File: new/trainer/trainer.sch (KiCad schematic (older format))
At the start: 14 parts

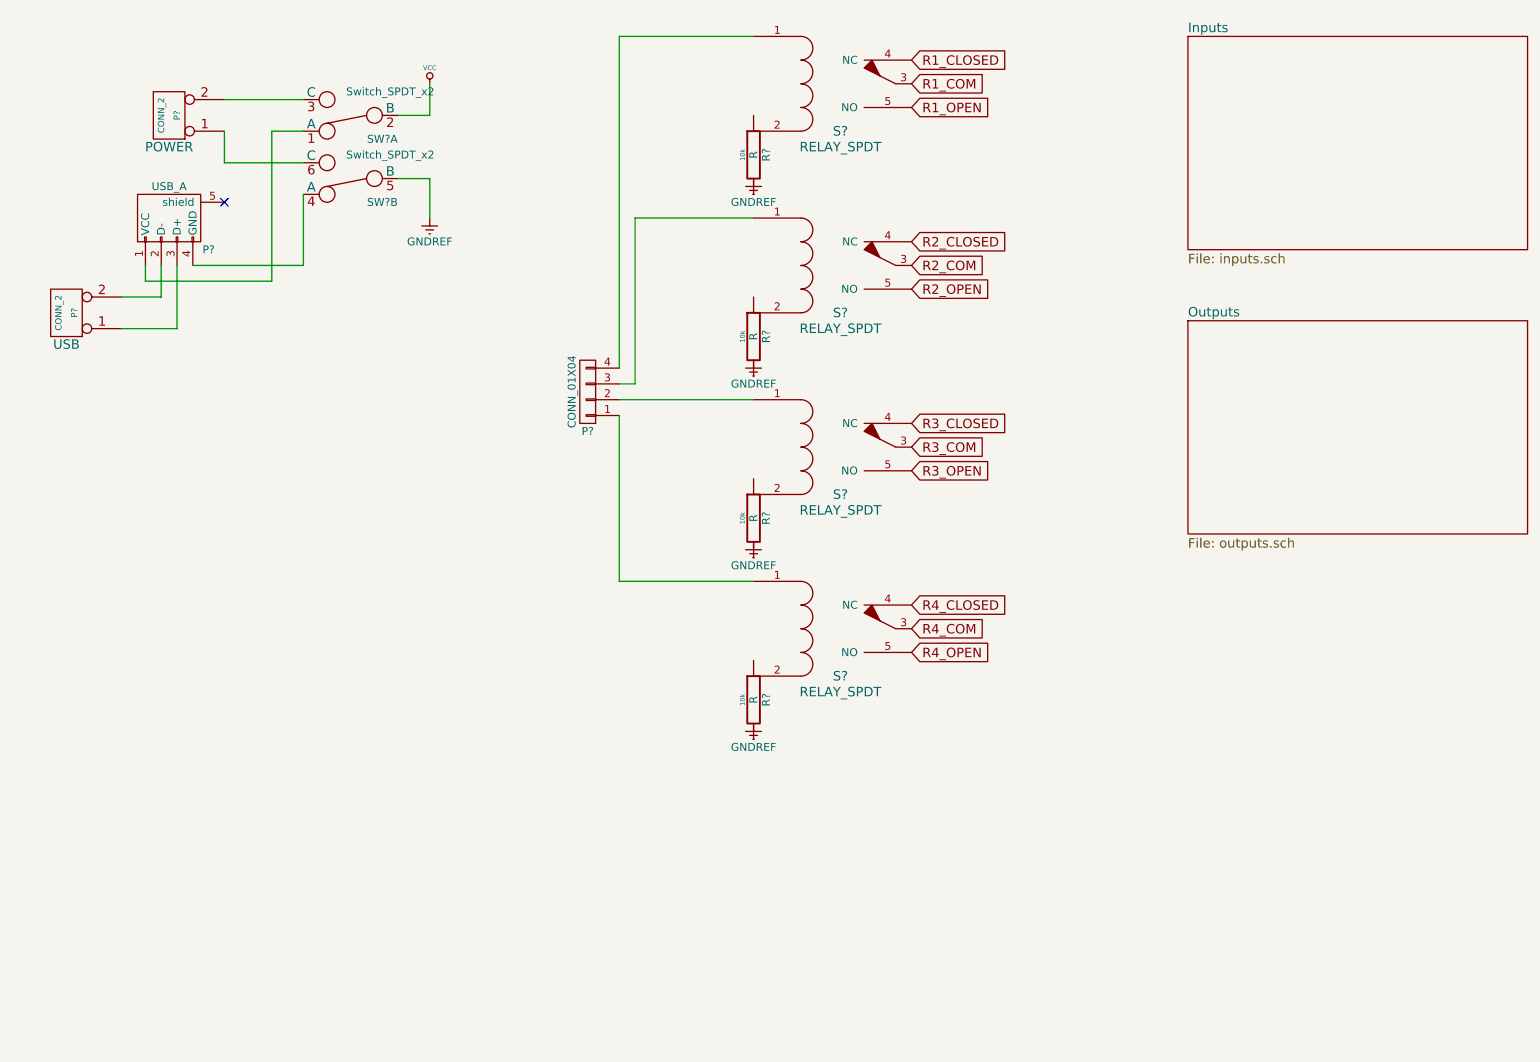
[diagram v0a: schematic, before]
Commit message: .
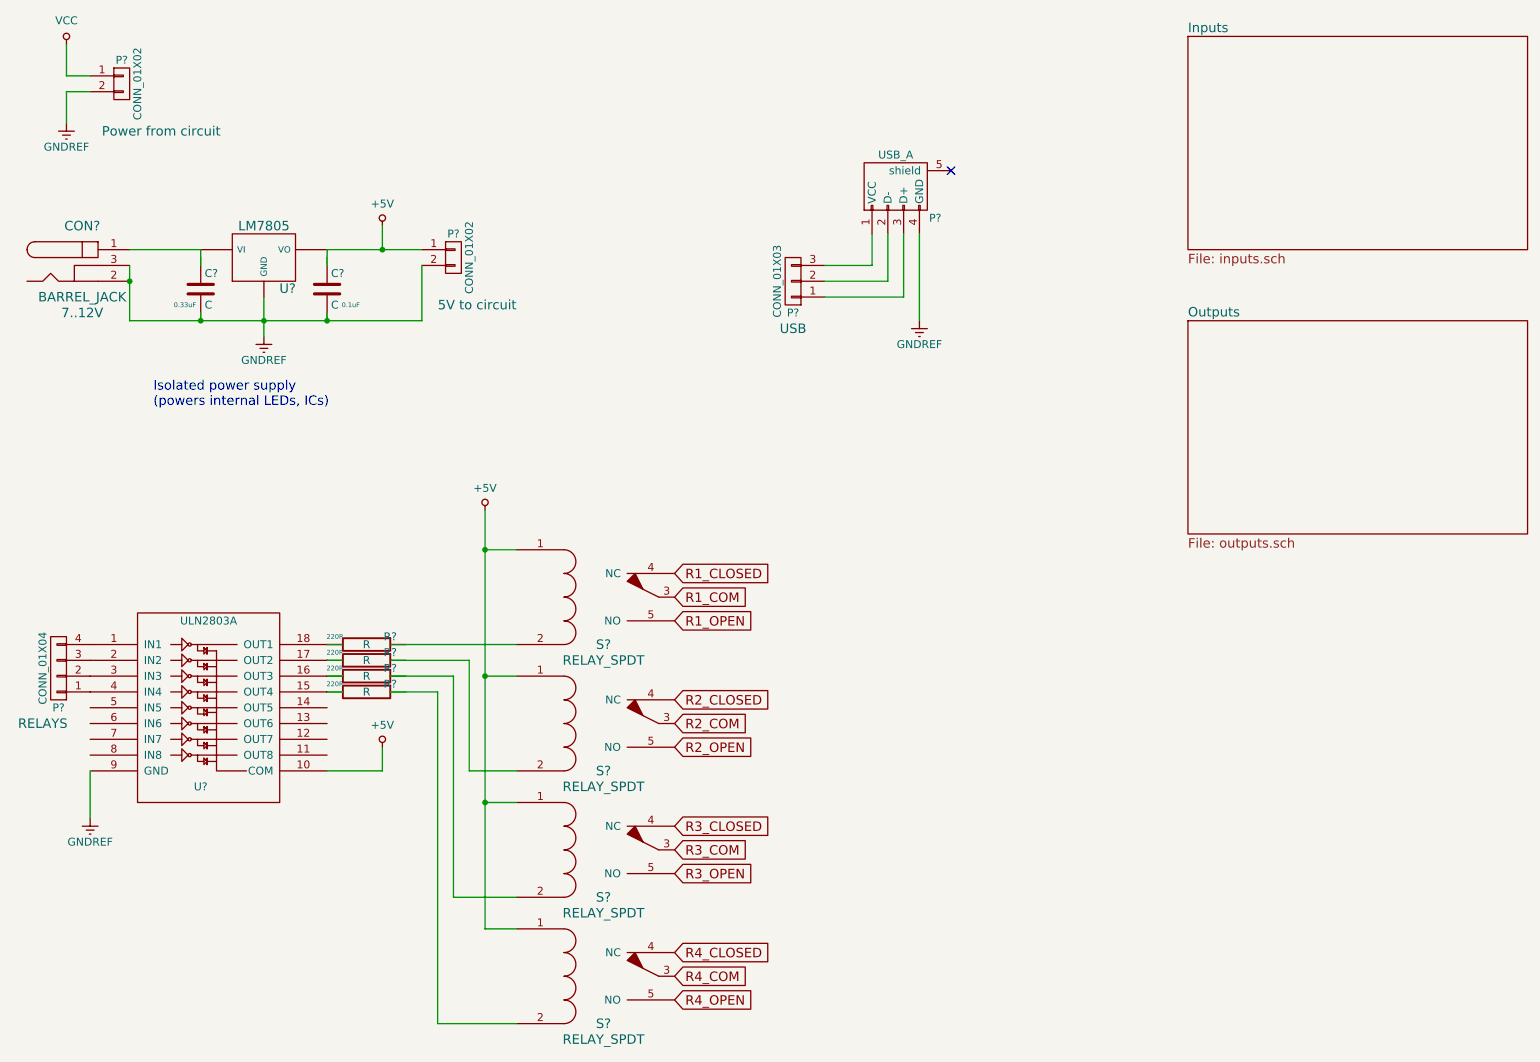
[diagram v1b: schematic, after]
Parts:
- removed P?: CONN_2, POWER, symbol CONN_2
- removed P?: CONN_2, USB, symbol CONN_2
- removed R? (x4): R, 10k, symbol R
- removed SW? (x2): Switch_SPDT_x2, symbol Switch_SPDT_x2
- added C?: C, 0.33uF, symbol C
- added C?: C, 0.1uF, symbol C
- added CON?: BARREL_JACK, 7..12V, symbol BARREL_JACK
- added P?: CONN_01X03, USB, symbol CONN_01X03
- added P?: CONN_01X02, 5V to circuit, symbol CONN_01X02
- added P?: CONN_01X02, Power from circuit, symbol CONN_01X02
- added R? (x4): R, 220R, symbol R
- added U?: LM7805, symbol LM7805
- added U?: ULN2803A, symbol ULN2803A
- P?: footprint (none) -> RELAYS
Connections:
- net labels added: +5V
- wire segments 25 -> 44
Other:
- note added: "Isolated power supply\n(powers internal LEDs, ICs)"
- moved on the sheet: P?, S?
